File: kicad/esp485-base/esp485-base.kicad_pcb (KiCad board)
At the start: 2 copper layers, 48.3 x 20.3 mm, 7 parts, among them J1 Conn_01x04, J2 Conn_02x06_Odd_Even, J3 Conn_01x07, J4 Conn_01x07, J5 Conn_01x03, U1 AMS1117-3.3

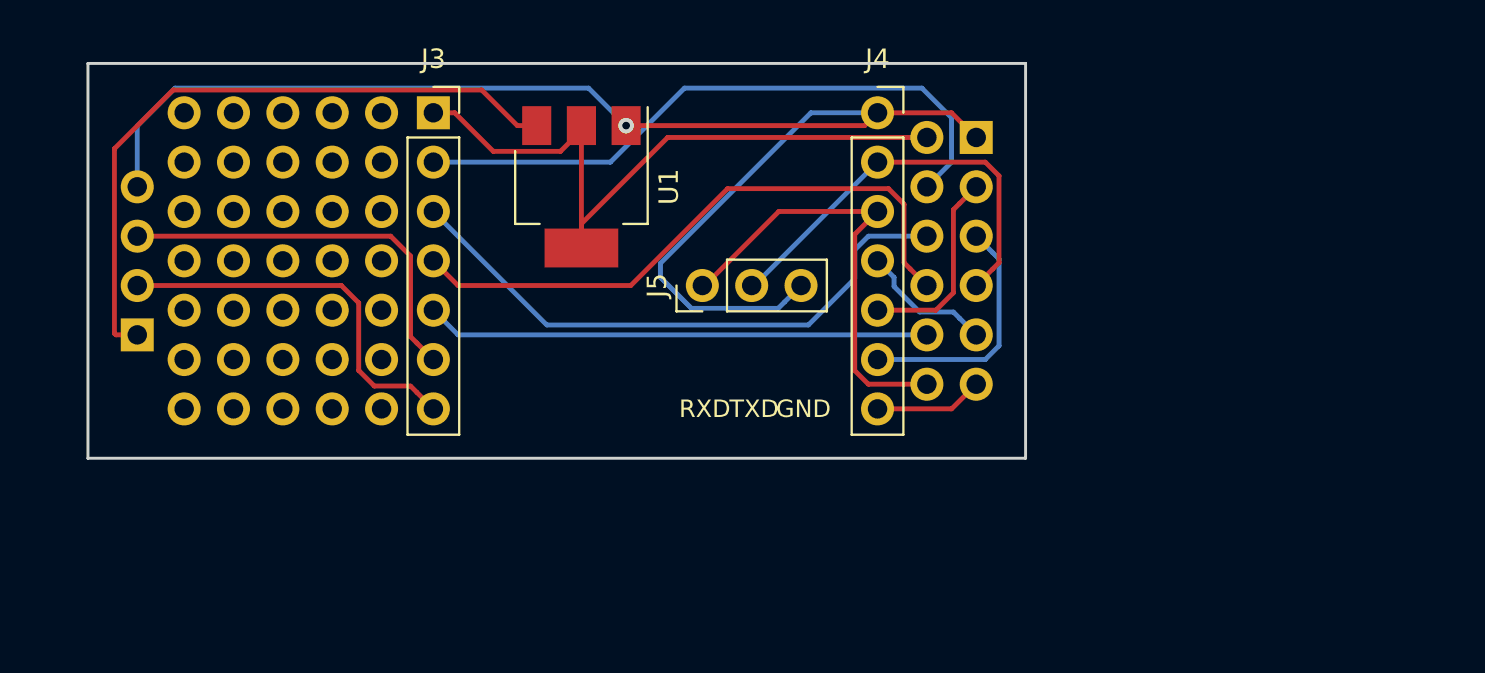
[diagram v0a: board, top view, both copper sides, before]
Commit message: esp485 base board
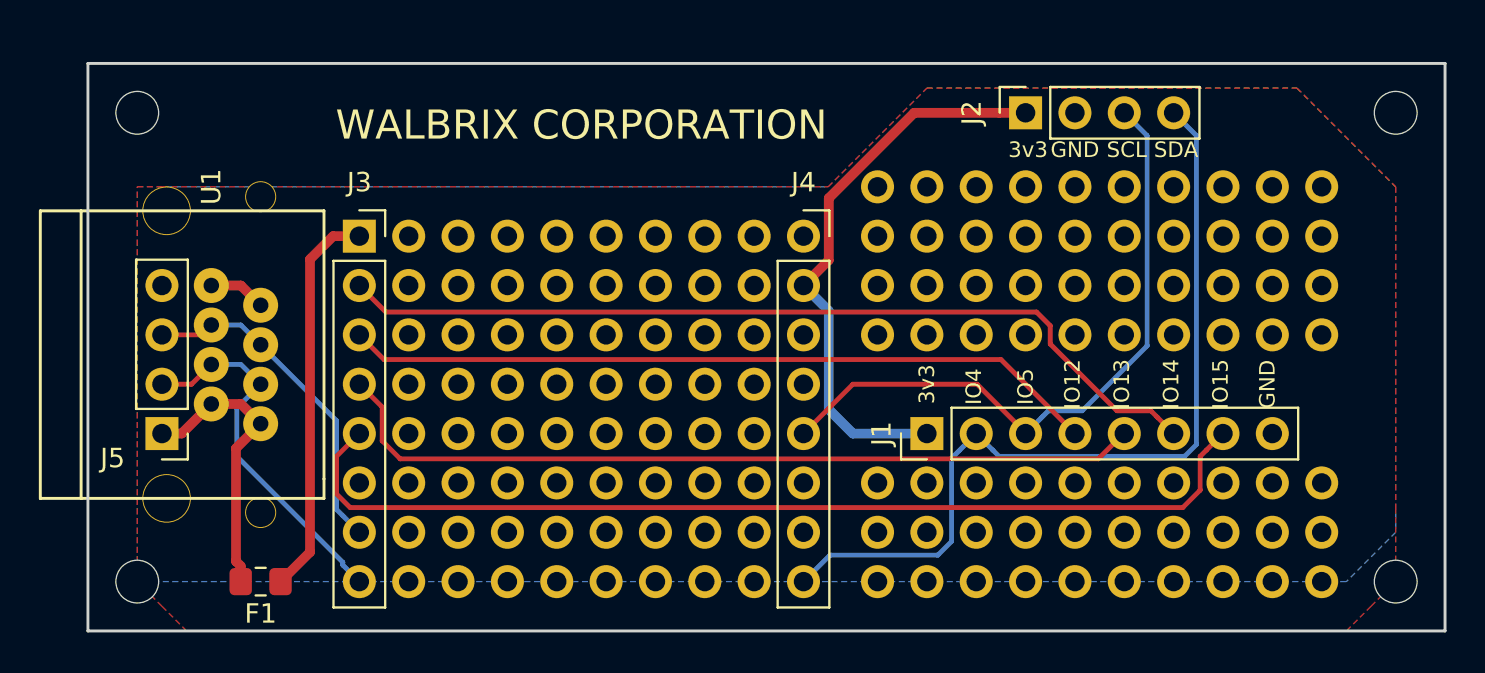
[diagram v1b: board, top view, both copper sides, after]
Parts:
- removed the REF** at (124.3, 100.3)
- added F1: Fuse, Fuse:Fuse_0805_2012Metric_Pad1.15x1.40mm_HandSolder, F.Cu at (123.2, 116.8)
- added REF**: MountingHole_2.2mm_M2, MountingHole:MountingHole_2.2mm_M2, F.Cu at (116.8, 92.7)
- added REF**: MountingHole_2.2mm_M2, MountingHole:MountingHole_2.2mm_M2, F.Cu at (181.6, 92.7)
- added REF**: MountingHole_2.2mm_M2, MountingHole:MountingHole_2.2mm_M2, F.Cu at (181.6, 116.8)
- added REF**: MountingHole_2.2mm_M2, MountingHole:MountingHole_2.2mm_M2, F.Cu at (116.8, 116.8)
- added REF**: prototype_area_8x8, lib:prototype_area_8x8, F.Cu at (139.7, 105.4)
- added REF**: prototype_area_10x4, lib:prototype_area_10x4, F.Cu at (166.4, 100.3)
- added REF**: prototype_area_10x3, lib:prototype_area_10x3, F.Cu at (166.4, 114.3)
- J1: value Conn_01x04 -> Conn_01x08; footprint Connector_PinHeader_2.54mm:PinHeader_1x04_P2.54mm_Vertical -> Connector_PinHeader_2.54mm:PinHeader_1x08_P2.54mm_Vertical; moved to F.Cu
- J2: value Conn_02x06_Odd_Even -> Conn_01x04; footprint Connector_PinHeader_2.54mm:PinHeader_2x06_P2.54mm_Vertical -> Connector_PinSocket_2.54mm:PinSocket_1x04_P2.54mm_Vertical; moved to F.Cu
- J3, J4: value Conn_01x07 -> Conn_01x08; footprint Connector_PinSocket_2.54mm:PinSocket_1x07_P2.54mm_Vertical -> Connector_PinSocket_2.54mm:PinSocket_1x08_P2.54mm_Vertical
- J5: value Conn_01x03 -> Conn_01x04; footprint Connector_PinHeader_2.54mm:PinHeader_1x03_P2.54mm_Vertical -> Connector_PinHeader_2.54mm:PinHeader_1x04_P2.54mm_Vertical
- U1: value AMS1117-3.3 -> 7810-8P8C; footprint Package_TO_SOT_SMD:SOT-223-3_TabPin2 -> 7810-8P8C:7810-8P8C
- moved J1 41.0 mm to (157.5, 109.2), turned to 90 degrees
- moved J5 28.8 mm to (118.1, 109.2), turned to 180 degrees
- moved U1 20.9 mm to (120.7, 105.2)
- moved J3 7.41 mm to (128.3, 99.1)
- moved J4 7.41 mm to (151.1, 99.1)
- moved J2 2.84 mm to (162.6, 92.7), turned to 90 degrees
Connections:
- J1 pad 1: VCC -> +3V3
- J1 pad 4: GND -> Net-(J1-Pad4)
- J2 pad 1: GND -> +3V3
- J2 pad 2: Net-(J2-Pad2) -> GND
- J2 pad 3: Net-(J2-Pad3) -> Net-(J1-Pad3)
- J2 pad 4: Net-(J2-Pad4) -> Net-(J1-Pad2)
- J3 pad 1: Net-(J2-Pad2) -> /VIN
- J3 pad 2: Net-(J2-Pad4) -> Net-(J1-Pad6)
- J3 pad 3: Net-(J2-Pad6) -> Net-(J1-Pad4)
- J3 pad 4: Net-(J2-Pad8) -> Net-(J1-Pad5)
- J3 pad 5: Net-(J2-Pad10) -> Net-(J1-Pad7)
- J3 pad 6: Net-(J1-Pad3) -> Net-(J3-Pad6)
- J3 pad 7: Net-(J1-Pad2) -> /A
- J4 pad 2: Net-(J2-Pad7) -> +3V3
- J4 pad 3: Net-(J2-Pad12) -> Net-(J4-Pad3)
- J4 pad 4: Net-(J2-Pad9) -> Net-(J4-Pad4)
- J4 pad 5: Net-(J2-Pad3) -> Net-(J1-Pad3)
- J4 pad 6: Net-(J2-Pad5) -> Net-(J4-Pad6)
- J4 pad 7: Net-(J2-Pad11) -> Net-(J4-Pad7)
- J5 pad 1: Net-(J2-Pad12) -> VCC
- J5 pad 2: Net-(J2-Pad7) -> /B
- J5 pad 3: GND -> /A
- U1 pad 1: GND -> VCC
- U1 pad 2: Net-(J2-Pad2) -> VCC
- U1 pad 3: VCC -> /B
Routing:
- net GND: track 72.2 -> 2.96 mm, vias 1 -> 0
- net Net-(J1-Pad7): track 0.00 -> 52.1 mm
- net Net-(J1-Pad6): track 0.00 -> 45.6 mm
- net Net-(J1-Pad5): track 0.00 -> 42.4 mm
- net Net-(J1-Pad4): track 0.00 -> 38.9 mm
- net Net-(J2-Pad2): track 36.3 -> 0.00 mm
- net Net-(J2-Pad4): track 33.0 -> 0.00 mm
- net Net-(J2-Pad8): track 31.8 -> 0.00 mm
- net Net-(J2-Pad6): track 30.6 -> 0.00 mm
- net +3V3: track 0.00 -> 29.5 mm
- net Net-(J2-Pad10): track 25.9 -> 0.00 mm
- net Net-(J1-Pad2): track 19.9 -> 44.2 mm
- net Net-(J2-Pad12): track 23.1 -> 0.00 mm
- net Net-(J2-Pad7): track 21.7 -> 0.00 mm
- net /VIN: track 0.00 -> 20.3 mm
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- added copper zone on B.Cu, net GND
- added copper zone on F.Cu, net GND
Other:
- board size 48.3 x 20.3 mm -> 69.9 x 29.2 mm
- net class Power added: clearance 0.2, trace_width 0.5, via_dia 0.8, via_drill 0.4
- board text added: "3v3"
- board text added: "A0"
- board text added: "IO0"
- board text added: "IO12"
- board text added: "IO13"
- board text added: "IO14"
- board text added: "IO15"
- board text added: "IO4"
- board text added: "IO5"
- board text added: "RST"
- board text added: "SCL"
- board text added: "SDA"
- board text added: "VIN"
- board text added: "WALBRIX CORPORATION"
